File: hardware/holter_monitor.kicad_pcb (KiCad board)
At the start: 2 copper layers, 70 x 90 mm, 52 parts, among them J1 USB_C_Receptacle_USB2.0_16P, J2 BAT JST-PH, J4 UART, Q1 AO3401A, SW1 SW_SPDT, SW2 RESET, SW3 BOOT, U1 USBLC6-2SC6, U2 MCP73831-2-OT, U3 AP2112K-3.3, U4 ESP32-S3-WROOM-1, U5 SEN-12650

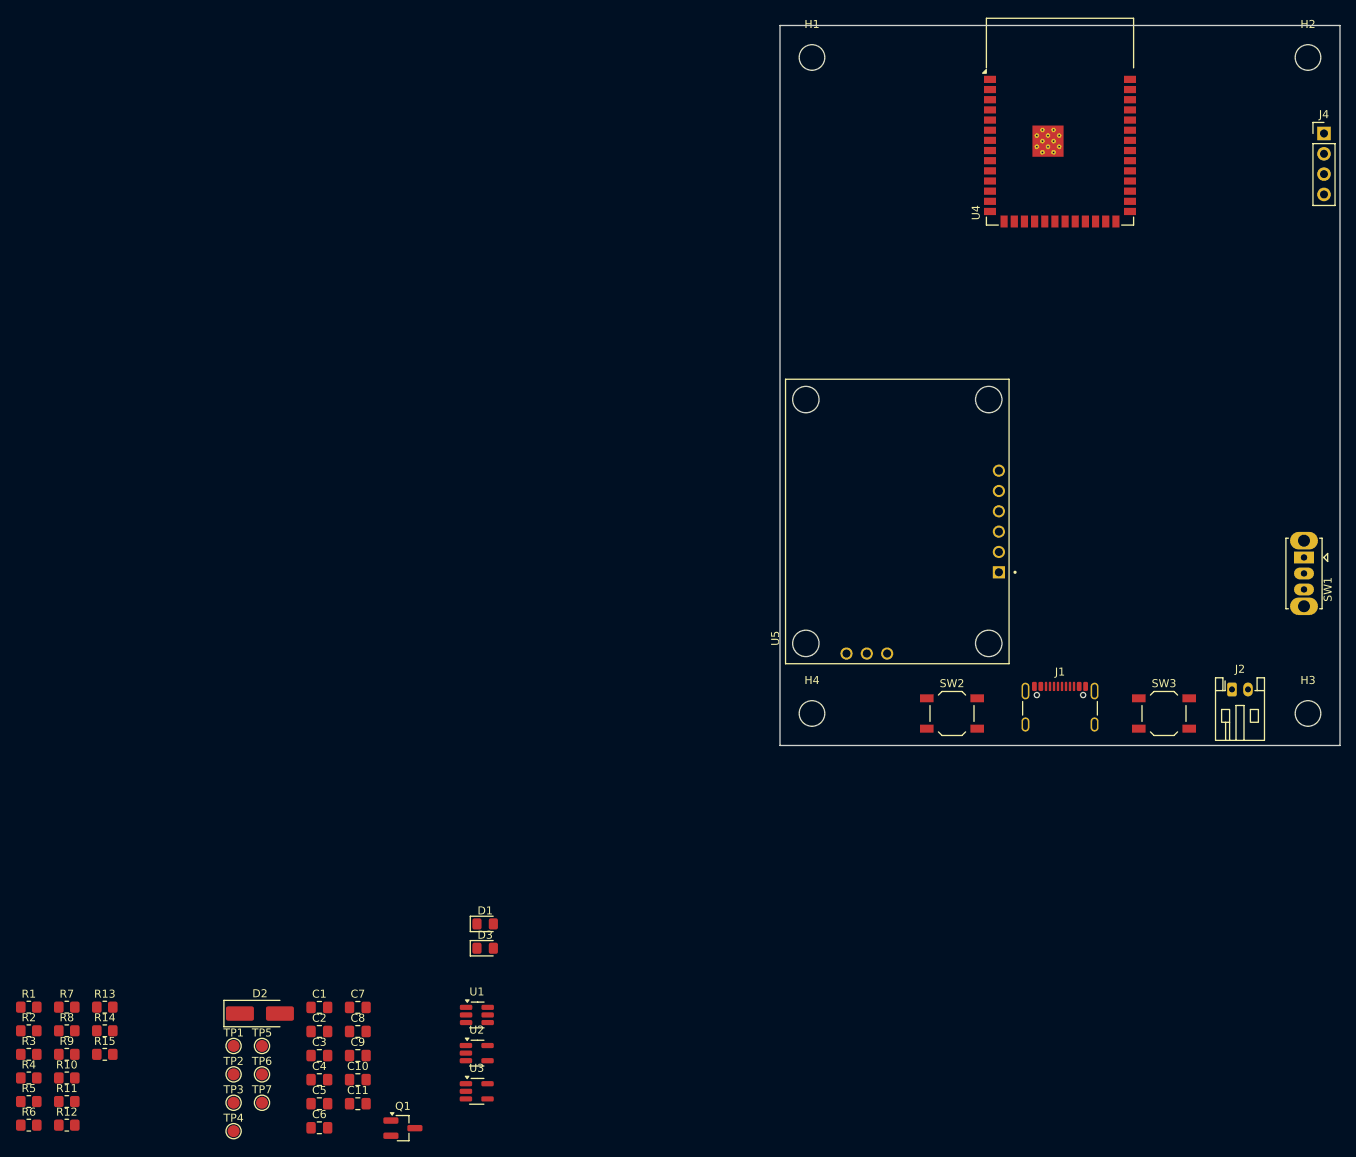
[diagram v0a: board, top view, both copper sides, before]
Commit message: Placed all of the elements on the board
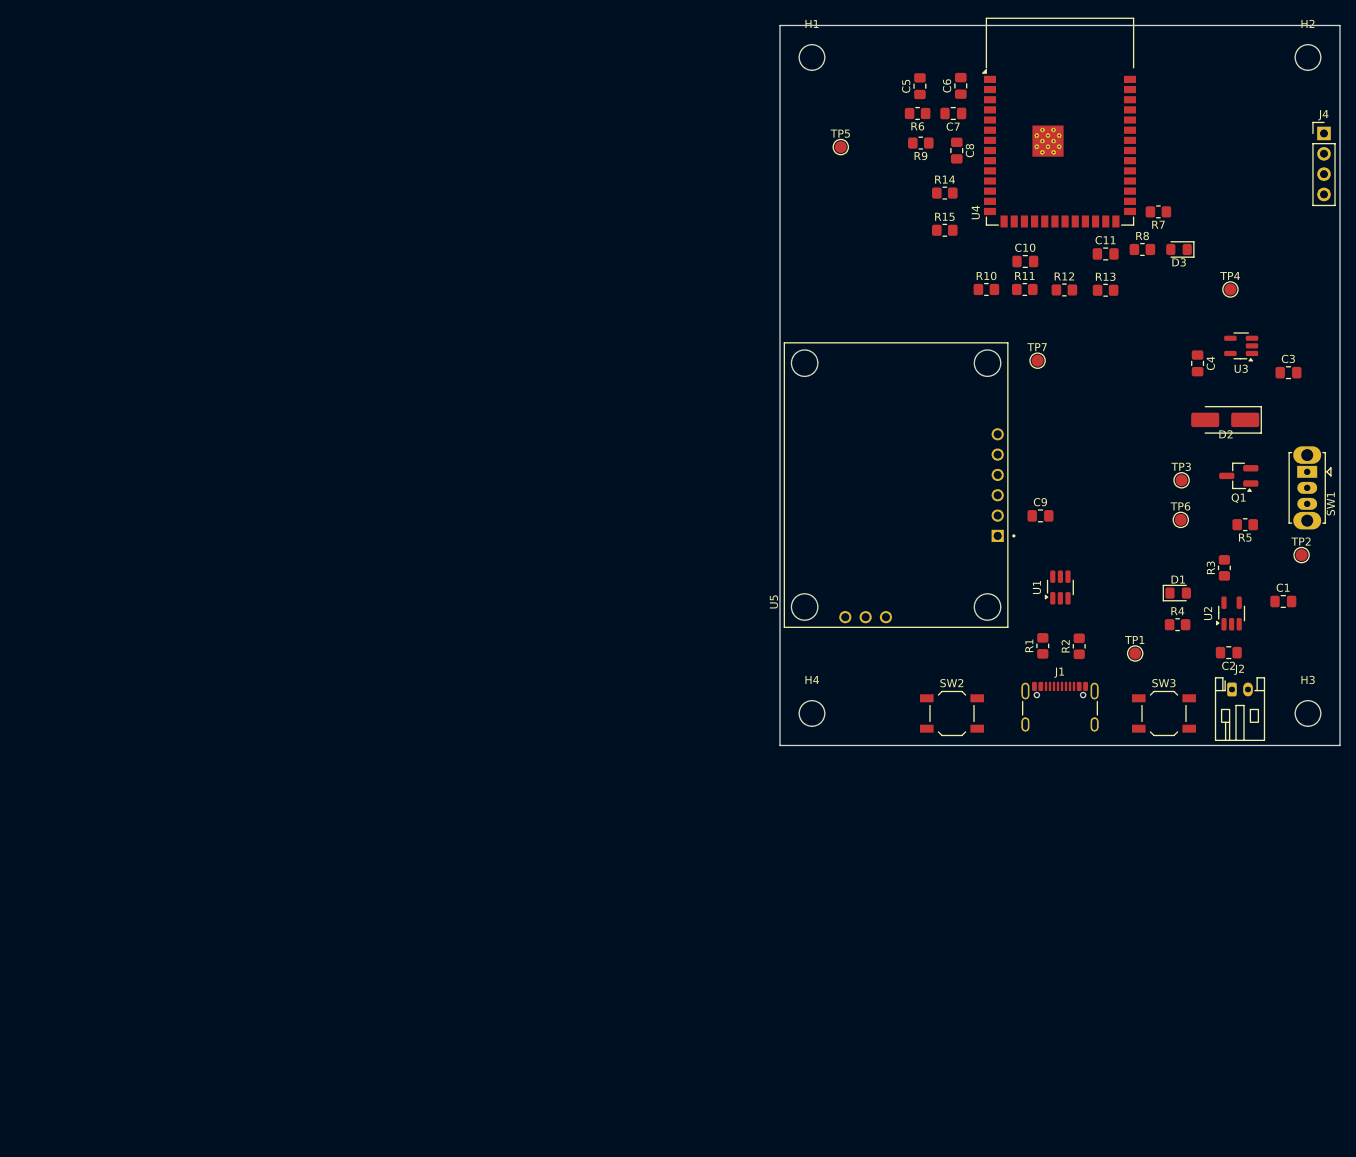
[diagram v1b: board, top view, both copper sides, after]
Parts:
- moved R7 168.8 mm to (162.3, 77.3), turned to 180 degrees
- moved R6 168.3 mm to (132.2, 65.0), turned to 180 degrees
- moved R5 168.3 mm to (173.2, 116.4), turned to 180 degrees
- moved R8 166.2 mm to (160.3, 82.0)
- moved TP4 163.1 mm to (171.3, 87.0)
- moved R12 162.6 mm to (150.6, 87.1)
- moved R3 161.3 mm to (170.6, 121.8), turned to 90 degrees
- moved R11 157.0 mm to (145.6, 87.0)
- moved R9 156.1 mm to (132.6, 68.7), turned to 180 degrees
- moved R4 154.4 mm to (164.7, 128.9)
- moved R13 153.9 mm to (155.7, 87.1)
- moved C6 152.9 mm to (137.6, 61.5), turned to 90 degrees
- moved R10 151.4 mm to (140.8, 87.0)
- moved TP2 148.4 mm to (180.2, 120.2)
- moved R14 148.3 mm to (135.6, 75.0)
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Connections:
- U4 pad 17: unconnected-(U4-IO9-Pad17) -> VBAT_SENSE
- U4 pad 18: unconnected-(U4-IO10-Pad18) -> VBUS_SENSE
- U4 pad 5: VBAT_SENSE -> unconnected-(U4-IO5-Pad5)
- U4 pad 6: VBUS_SENSE -> unconnected-(U4-IO6-Pad6)
